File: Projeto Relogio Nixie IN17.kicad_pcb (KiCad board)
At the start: 2 copper layers, 49.8 x 67.6 mm, 66 parts, among them J1 Conn_01x04, J2 Conn_02x12_Odd_Even, J3 Conn_01x24, J4 BATTERY, J5 ANTENNA, Q1 BC817, Q2 STD17NF25, Q3 BC817, Q4 BC548, Q5 BC548, Q6 BC548, SW1 SW_Push, SW2 SW_Push, SW3 SPST_B3U-1000P, SW4 SPST_B3U-1000P, U1 MAX1771xSA, U2 CP2102N-A01-GQFN24, U3 HV5523K7-G, U4 PAM2305AABADJ, U5 MCP73831-3-OT, U6 ESP32-PICO-D4

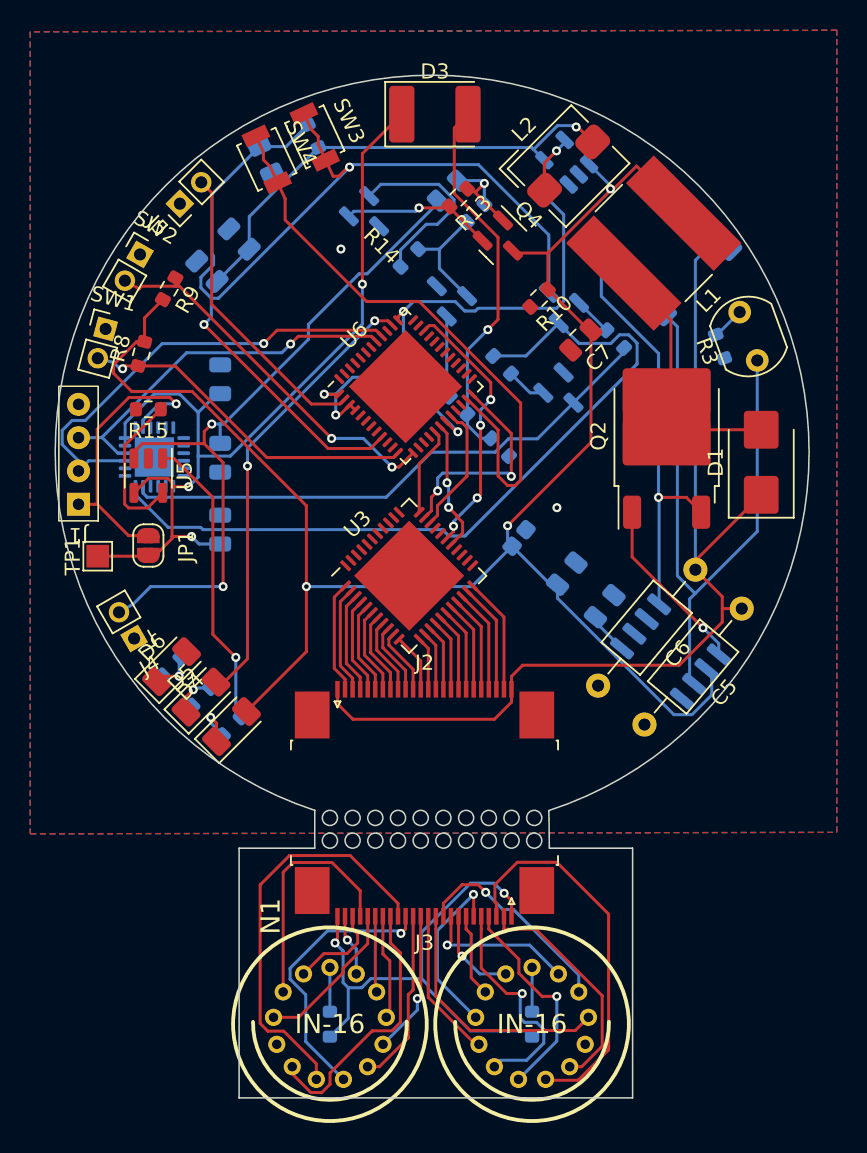
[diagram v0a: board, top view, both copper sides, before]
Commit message: Add files via upload
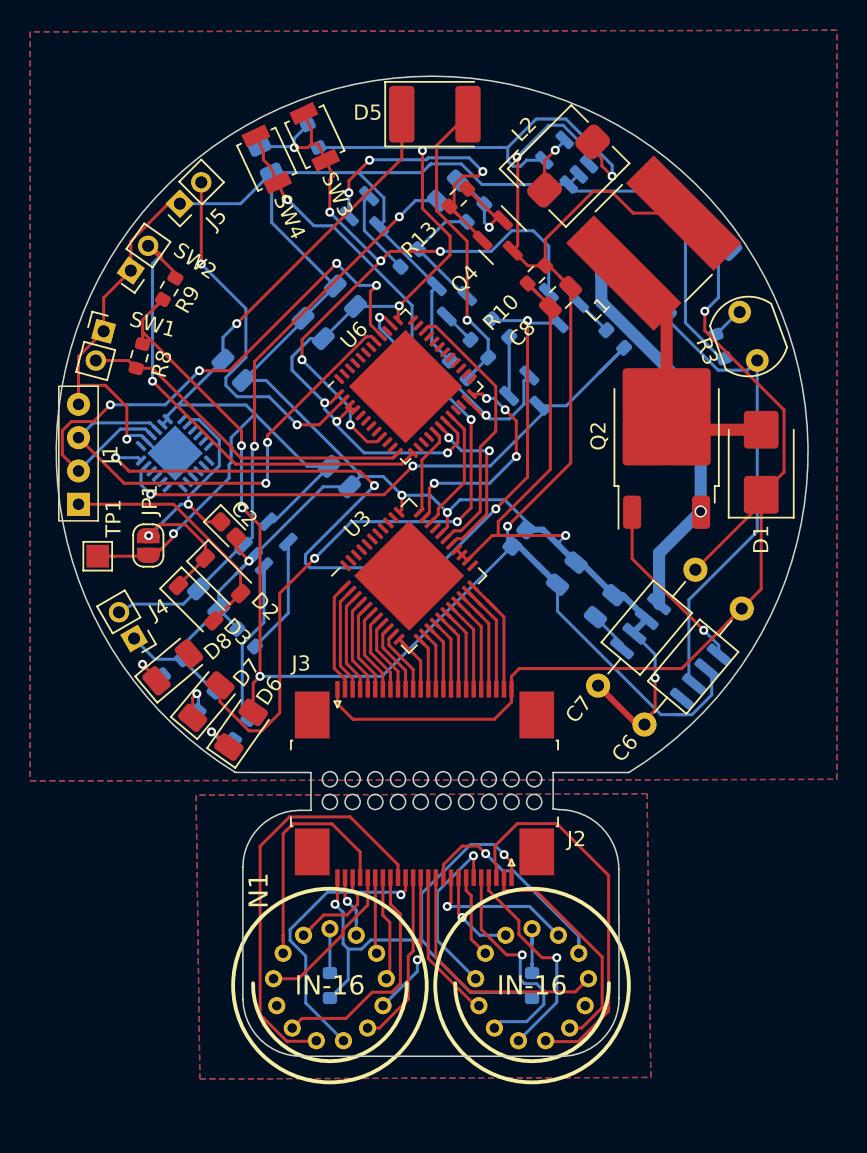
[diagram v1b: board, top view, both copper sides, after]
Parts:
- added C2: 100uF, Capacitor_Tantalum_SMD:CP_EIA-1608-08_AVX-J, F.Cu at (129.8, 66.9)
- added D2: 1N4148W, Diode_SMD:D_SOD-123, F.Cu at (129.4, 70.0)
- added D3: 1N4148W, Diode_SMD:D_SOD-123, F.Cu at (127.7, 71.8)
- R15, U5: moved to B.Cu
- moved R15 16.4 mm to (131.0, 74.1), turned to 135 degrees
- moved C1 10.6 mm to (130.1, 56.4), turned to -45 degrees
- moved C10 10.2 mm to (137.1, 63.4), turned to -45 degrees
- moved C9 9.37 mm to (128.5, 71.5), turned to -45 degrees
- moved U5 8.99 mm to (132.3, 67.9), turned to 45 degrees
- moved C11 7.98 mm to (137.5, 51.5)
- moved C12 7.98 mm to (135.4, 53.7)
- moved R17 5.82 mm to (145.0, 56.4), turned to -45 degrees
- moved R16 4.00 mm to (146.4, 55.0)
- moved C8 3.11 mm to (151.7, 51.6)
- moved J2 2.55 mm to (142.8, 88.6)
- moved N1 2.55 mm to (136.5, 97.1)
- moved N2 2.55 mm to (149.9, 97.1)
- moved R11 2.55 mm to (149.9, 97.1)
- moved R5 2.55 mm to (136.5, 97.1)
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- renumbered C9 to C10, C10 to C11, C11 to C12, C12 to C13, C2 to C3, C3 to C4, C4 to C5, C5 to C6, C6 to C7, C7 to C8, C8 to C9, D2 to D4, D3 to D5, D4 to D6, D5 to D7, D6 to D8, J3 to J2, J2 to J3
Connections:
- J1 pad 1: VIN -> Net-(D2-A)
- Q3 pad 2: IO0 -> BOOT
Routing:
- net BAT-: track 0.00 -> 217.7 mm, vias 2 -> 6
- net EN: track 70.9 -> 49.9 mm, vias 2 -> 6
- net Net-(D2-A): track 0.00 -> 16.6 mm
- net WIFI_LED: track 29.9 -> 45.4 mm, vias 2 -> 4
- net DCDC: track 114.0 -> 128.7 mm, vias 3 -> 5
- net FB: track 43.7 -> 32.5 mm
- net Net-(Q4-B): track 10.1 -> 19.7 mm, vias 1 -> 3
- net RX0: track 30.3 -> 39.3 mm, vias 1 -> 4
- net SW2: track 25.1 -> 33.8 mm, vias 2 -> 1
- net TX0: track 24.6 -> 33.0 mm, vias 1 -> 2
- net BAT+: track 47.3 -> 39.0 mm
- net BOOT: track 39.6 -> 32.0 mm, vias 0 -> 2
- net STAT: track 19.7 -> 12.7 mm, vias 1 -> 0
- net Net-(Q5-B): track 12.7 -> 5.80 mm
- net RST: track 52.3 -> 58.8 mm, vias 0 -> 4
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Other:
- board size 49.8 x 67.6 mm -> 49.7 x 64.8 mm
